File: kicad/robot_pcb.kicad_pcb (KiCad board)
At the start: 2 copper layers, 65.4 x 66 mm, 31 parts, among them J1 Conn_01x19_Female, J2 Conn_01x19_Female, J3 esp32 cam, J4 motor1, J5 motor2, J6 motor pwr, J7 esp32 pwr, Q1 Q_PMOS_GDS, Q2 Q_NMOS_GDS, Q3 Q_PMOS_GDS, Q4 Q_NMOS_GDS, Q5 Q_PMOS_GDS, Q6 Q_NMOS_GDS, Q7 Q_PMOS_GDS, Q8 Q_NMOS_GDS, U1 4N25, U2 4N25, U3 4N25, U4 4N25

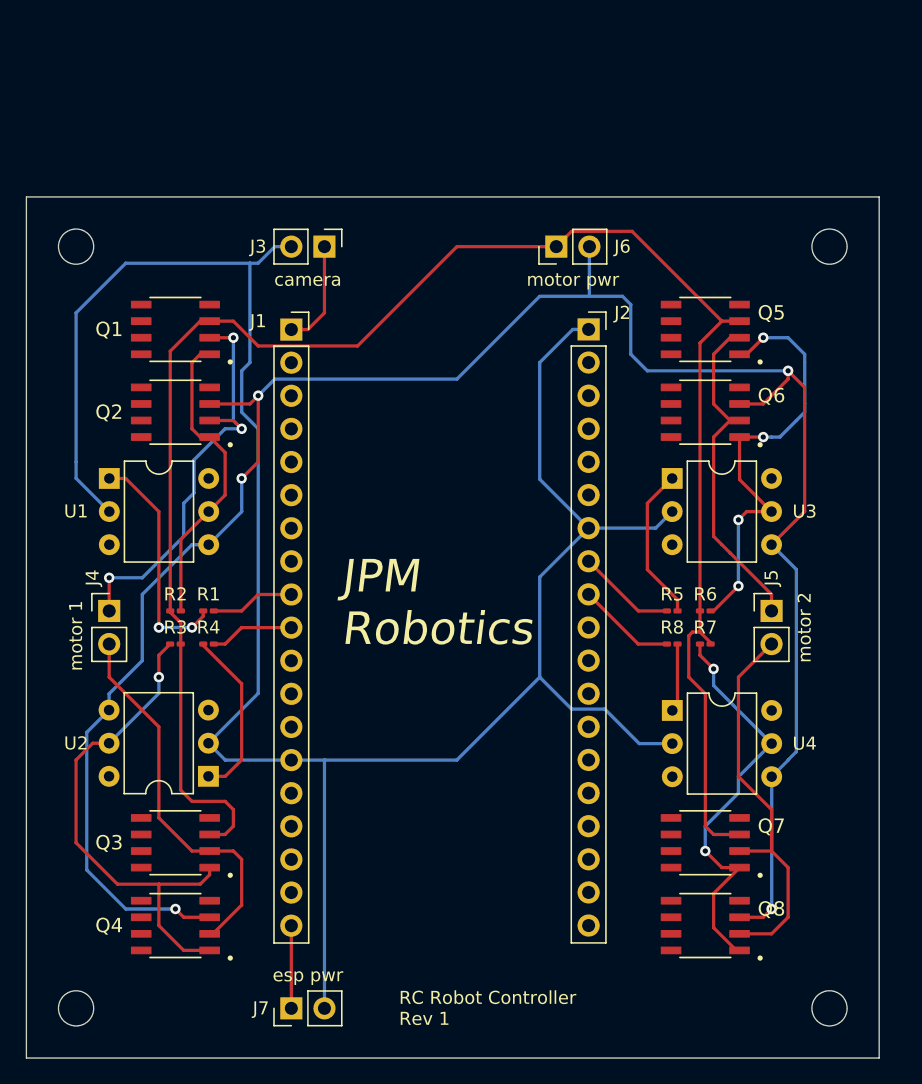
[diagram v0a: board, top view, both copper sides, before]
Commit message: add measurements kicad
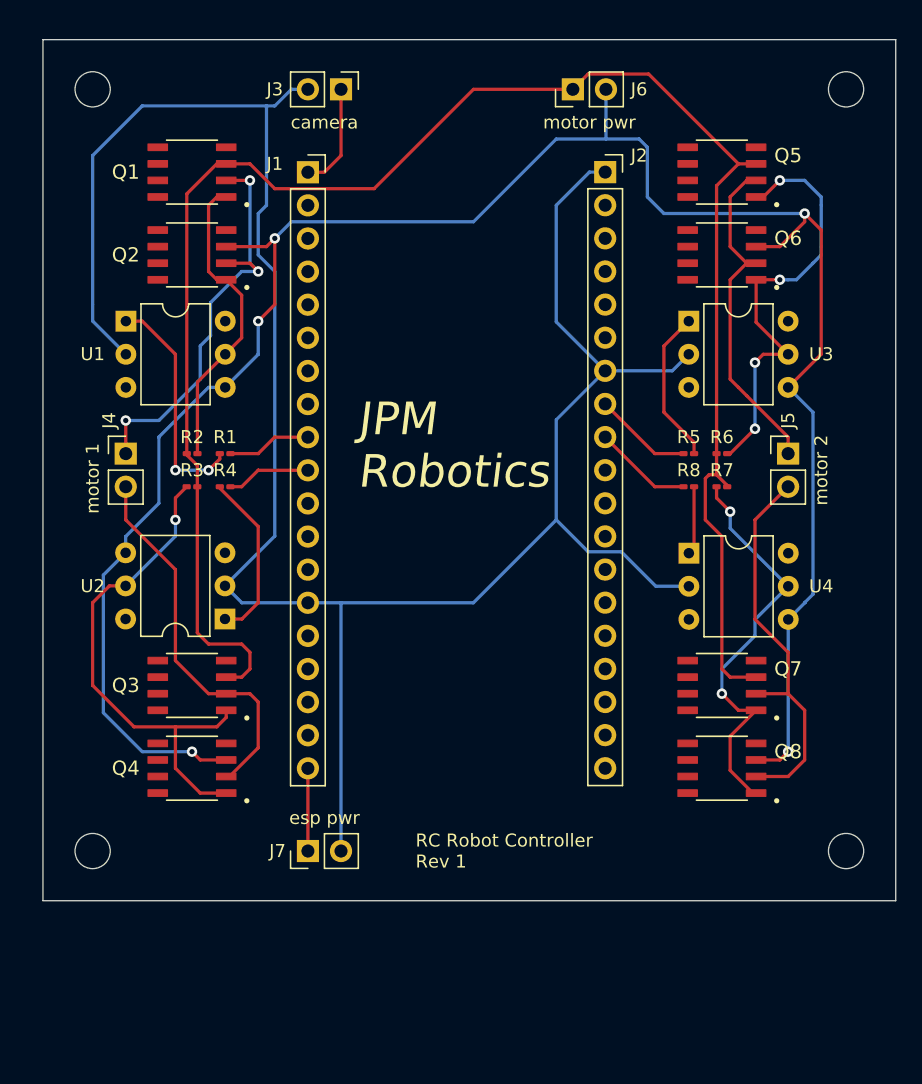
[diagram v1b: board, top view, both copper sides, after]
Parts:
- moved J5 12.1 mm to (149.9, 76.8)
- moved Q7 12.1 mm to (144.8, 94.6)
- moved R1 12.1 mm to (106.7, 76.8)
- moved R2 12.1 mm to (104.2, 76.8)
- moved R5 12.1 mm to (142.2, 76.8)
- moved R6 12.1 mm to (144.8, 76.8)
- moved J4 12.1 mm to (99.1, 76.8)
- moved Q3 12.1 mm to (104.1, 94.6)
- moved J2 12.1 mm to (135.8, 55.2)
- moved Q5 12.1 mm to (144.8, 55.2)
- moved Q1 12.1 mm to (104.1, 55.2)
- moved Q6 12.1 mm to (144.8, 61.6)
- moved Q8 12.1 mm to (144.8, 101.0)
- moved R4 12.1 mm to (106.7, 79.4)
- moved R7 12.1 mm to (144.8, 79.4)
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
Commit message: pcb rev 2
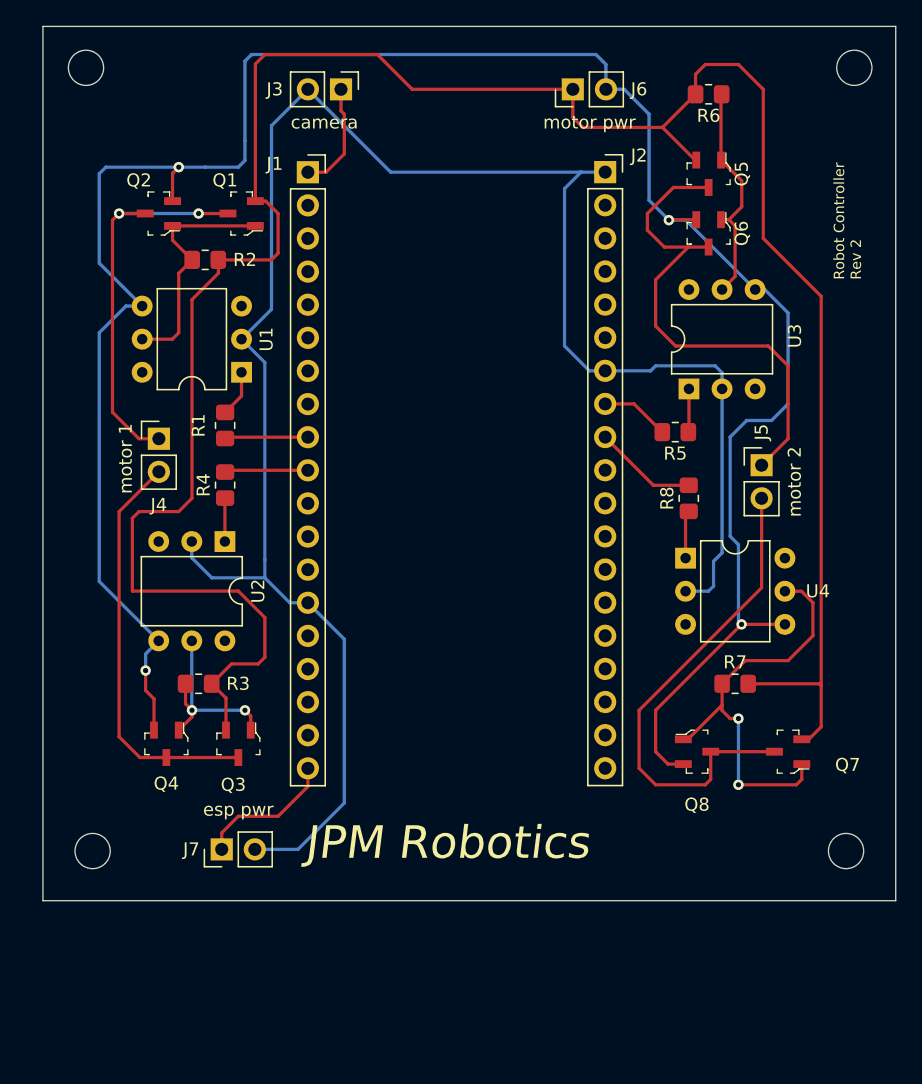
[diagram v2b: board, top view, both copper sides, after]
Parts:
- Q1, Q3, Q5, Q7: value Q_PMOS_GDS -> AO3401A; footprint Downloads:SOIC127P490X600X175-8N -> digikey-footprints:SOT-23-3
- Q2, Q4, Q6, Q8: value Q_NMOS_GDS -> IRLML6344TRPBF; footprint Downloads:SOIC127P490X600X175-8N -> digikey-footprints:SOT-23-3
- R1, R2, R3, R4, R5, R6, R7, R8: footprint Resistor_SMD:R_0201_0603Metric_Pad0.64x0.40mm_HandSolder -> Resistor_SMD:R_0805_2012Metric_Pad1.20x1.40mm_HandSolder
- moved R6 27.6 mm to (143.8, 49.3)
- moved R7 15.1 mm to (145.8, 94.5)
- moved R3 15.1 mm to (104.6, 94.5)
- moved R2 14.9 mm to (105.2, 62.0), turned to 0 degrees
- moved U1 9.70 mm to (107.9, 70.6), turned to 180 degrees
- moved Q7 7.18 mm to (149.9, 99.7)
- moved J7 6.61 mm to (106.4, 107.2)
- moved U2 5.94 mm to (106.7, 83.6), turned to -90 degrees
- moved Q3 5.72 mm to (107.7, 99.1), turned to -90 degrees
- moved U3 5.20 mm to (142.3, 71.9), turned to 90 degrees
- moved Q1 4.96 mm to (108.0, 58.4)
- moved Q2 4.07 mm to (101.6, 58.4)
- moved J4 2.79 mm to (101.6, 75.7)
- moved Q4 2.71 mm to (102.2, 99.1), turned to -90 degrees
- moved Q8 2.29 mm to (142.9, 99.7), turned to 0 degrees
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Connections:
- Q1 pad 2: MO1 -> /Vm
- Q1 pad 3: /Vm -> MO1
- Q2 pad 2: MO1 -> MGND
- Q2 pad 3: MGND -> MO1
- Q3 pad 2: MO2 -> /Vm
- Q3 pad 3: /Vm -> MO2
- Q4 pad 2: MO2 -> MGND
- Q4 pad 3: MGND -> MO2
- Q5 pad 2: MO3 -> /Vm
- Q5 pad 3: /Vm -> MO3
- Q6 pad 2: MO3 -> MGND
- Q6 pad 3: MGND -> MO3
- Q7 pad 2: MO4 -> /Vm
- Q7 pad 3: /Vm -> MO4
- Q8 pad 2: MO4 -> MGND
- Q8 pad 3: MGND -> MO4
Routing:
- net /Vm: track 138.7 -> 181.8 mm
- net ESP_GND: track 173.0 -> 148.2 mm
- net /Gate2: track 39.2 -> 15.3 mm, vias 1 -> 2
- net /Gate3: track 33.8 -> 17.3 mm, vias 4 -> 0
- net Net-(R1-Pad1): track 17.9 -> 3.60 mm, vias 2 -> 0
- net MO3: track 25.8 -> 39.0 mm
- net MGND: track 162.0 -> 173.4 mm, vias 5 -> 4
- net Net-(R4-Pad1): track 13.2 -> 3.33 mm
- net Net-(R5-Pad1): track 11.9 -> 3.33 mm
- net MO4: track 30.3 -> 37.8 mm
- net /Gate1: track 23.5 -> 18.6 mm
- net /Vcc: track 6.34 -> 10.7 mm
- net M21: track 7.58 -> 5.27 mm
- net MO1: track 32.2 -> 30.2 mm, vias 3 -> 2
- net MO2: track 29.5 -> 31.4 mm
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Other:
- board size 65.4 x 66 mm -> 65.4 x 67.1 mm
- board text added: "Robot Controller Rev 2"
- board text removed: "RC Robot Controller Rev 1"
